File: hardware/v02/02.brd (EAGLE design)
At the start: 88.6 x 50.8 mm, 33 parts, among them IC1 MSP430G2553, IC2 78L05Z, X2 RJ45-6L-B

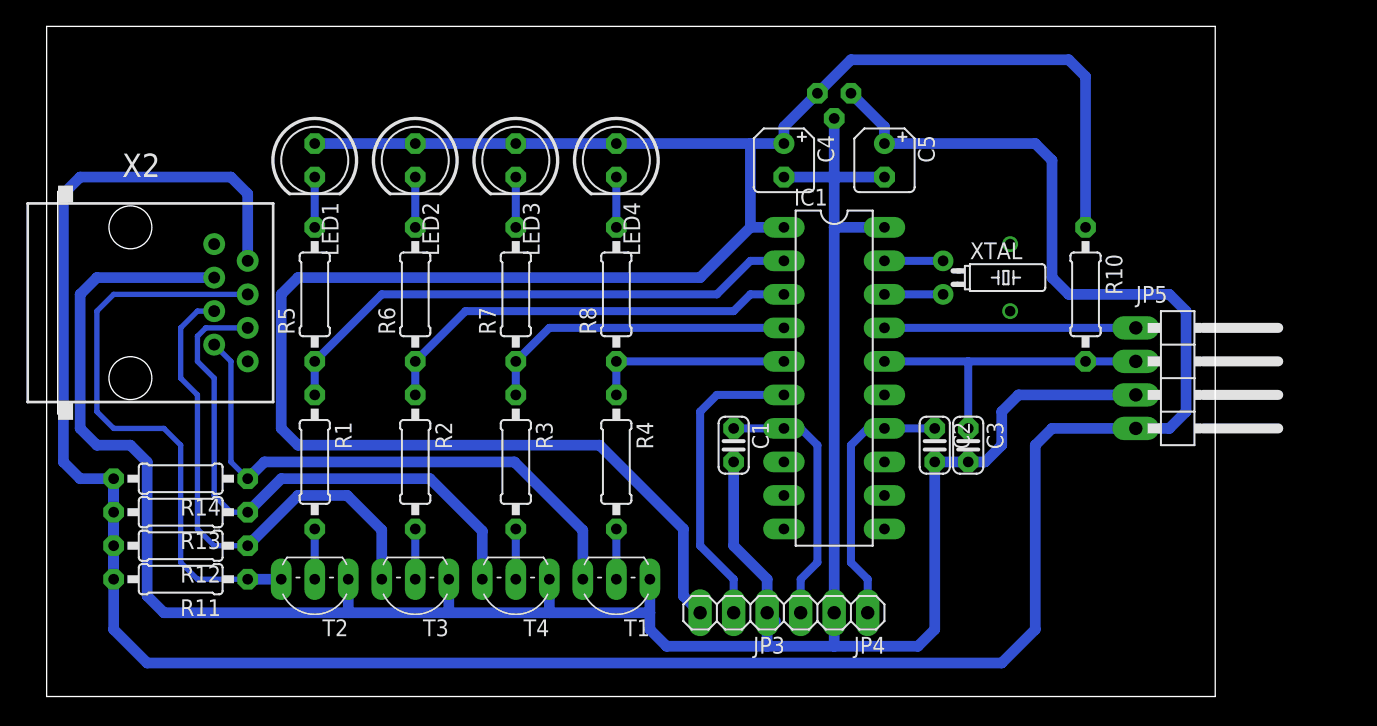
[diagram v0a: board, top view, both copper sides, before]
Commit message: rearrange
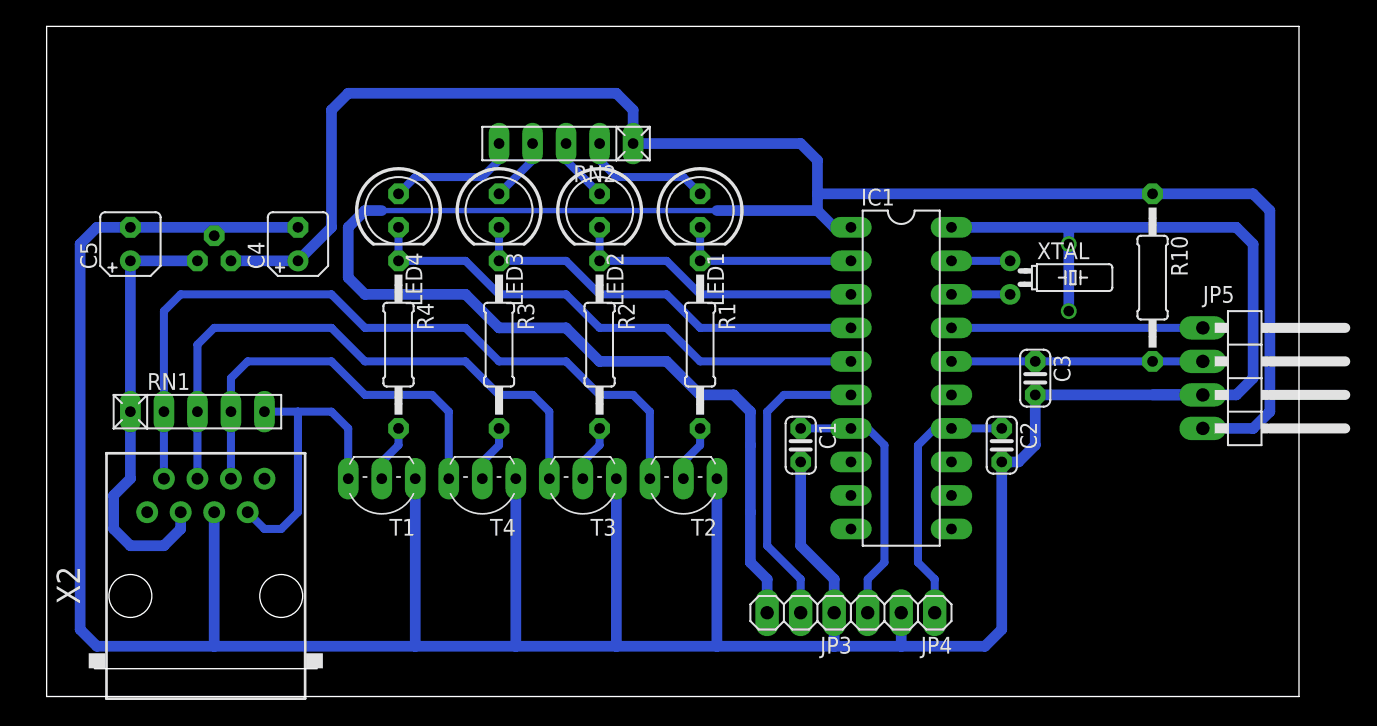
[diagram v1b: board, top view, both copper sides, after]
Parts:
- removed R11, R12, R13, R14: 10k, rcl:0207/10
- removed R5, R6, R7, R8: 220, rcl:0207/10
- added RN1: 4.7k, resistor-net:RN-5
- added RN2: 220, resistor-net:RN-5
- R1, R10, R2, R3, R4: device rcl:0207/10 -> rcl:0207/12
- moved C5 57.5 mm to (6.35, 34.3), turned to 90 degrees
- moved IC2 48.7 mm to (12.7, 33.0), turned to 0 degrees
- moved C4 37.4 mm to (19.1, 34.3), turned to 90 degrees
- moved R1 30.5 mm to (49.5, 26.7)
- moved LED1 29.5 mm to (49.5, 36.8)
- moved T2 29.0 mm to (48.3, 15.2)
- moved X2 22.9 mm to (12.1, 7.62), turned to 0 degrees
- moved T1 19.3 mm to (25.4, 15.2)
- moved R4 18.8 mm to (26.7, 26.7)
- moved LED4 16.9 mm to (26.7, 36.8)
- moved R2 16.6 mm to (41.9, 26.7)
- moved T3 14.8 mm to (40.6, 15.2)
- moved LED2 14.5 mm to (41.9, 36.8)
- moved R3 8.98 mm to (34.3, 26.7)
- moved T4 8.03 mm to (33.0, 15.2)
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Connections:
- removed net N$17: LED2.K, R6.2
- removed net N$21: LED3.K, R7.2
- new net N$10: LED2.A, RN2.3
- new net N$14: LED4.A, RN2.5
- net +5V: now also RN1.1, X2.3; no longer JP5.4, R11.2, R12.2, R13.2, R14.2, X2.2
- net GND: now also X2.5; no longer X2.3
- net N$12: now also LED1.K; no longer R5.1
- net N$13: now also LED3.A, RN2.4; no longer LED1.K, R5.2
- net N$8: now also LED1.A, RN2.2; no longer LED4.K, R8.2
- net N$9: now also LED2.K; no longer R6.1
- net OUT1: now also RN1.2, X2.2; no longer R11.1, X2.4
- net OUT2: now also RN1.3, X2.4; no longer R12.1, X2.5
- net OUT3: now also RN1.4; no longer R13.1
- net OUT4: now also RN1.5; no longer R14.1
- net PB: now also LED4.K; no longer R8.1
- net PR: now also LED3.K; no longer R7.1
- net VCC: now also JP5.4, RN2.1; no longer LED1.A, LED2.A, LED3.A, LED4.A
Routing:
- net +5V: track 208.0 -> 33.3 mm
- net GND: track 208.7 -> 276.6 mm, vias 0 -> 2
- net VCC: track 171.0 -> 211.4 mm
- net N$12: track 41.3 -> 14.0 mm
- net PB: track 15.2 -> 40.0 mm
- net OUT4: track 43.0 -> 23.2 mm
- net OUT1: track 44.0 -> 58.8 mm
- net OUT3: track 43.9 -> 31.3 mm
- net N$9: track 32.6 -> 22.6 mm
- net N$14: track 0.00 -> 9.94 mm
- net PR: track 23.9 -> 31.3 mm
- net N$8: track 3.81 -> 9.94 mm
- net OUT2: track 39.7 -> 45.1 mm
- net N$5: track 24.1 -> 19.0 mm
- net N$10: track 0.00 -> 4.86 mm
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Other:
- board size 88.6 x 50.8 mm -> 94.9 x 50.8 mm
